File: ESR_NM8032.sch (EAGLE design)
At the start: 68 parts

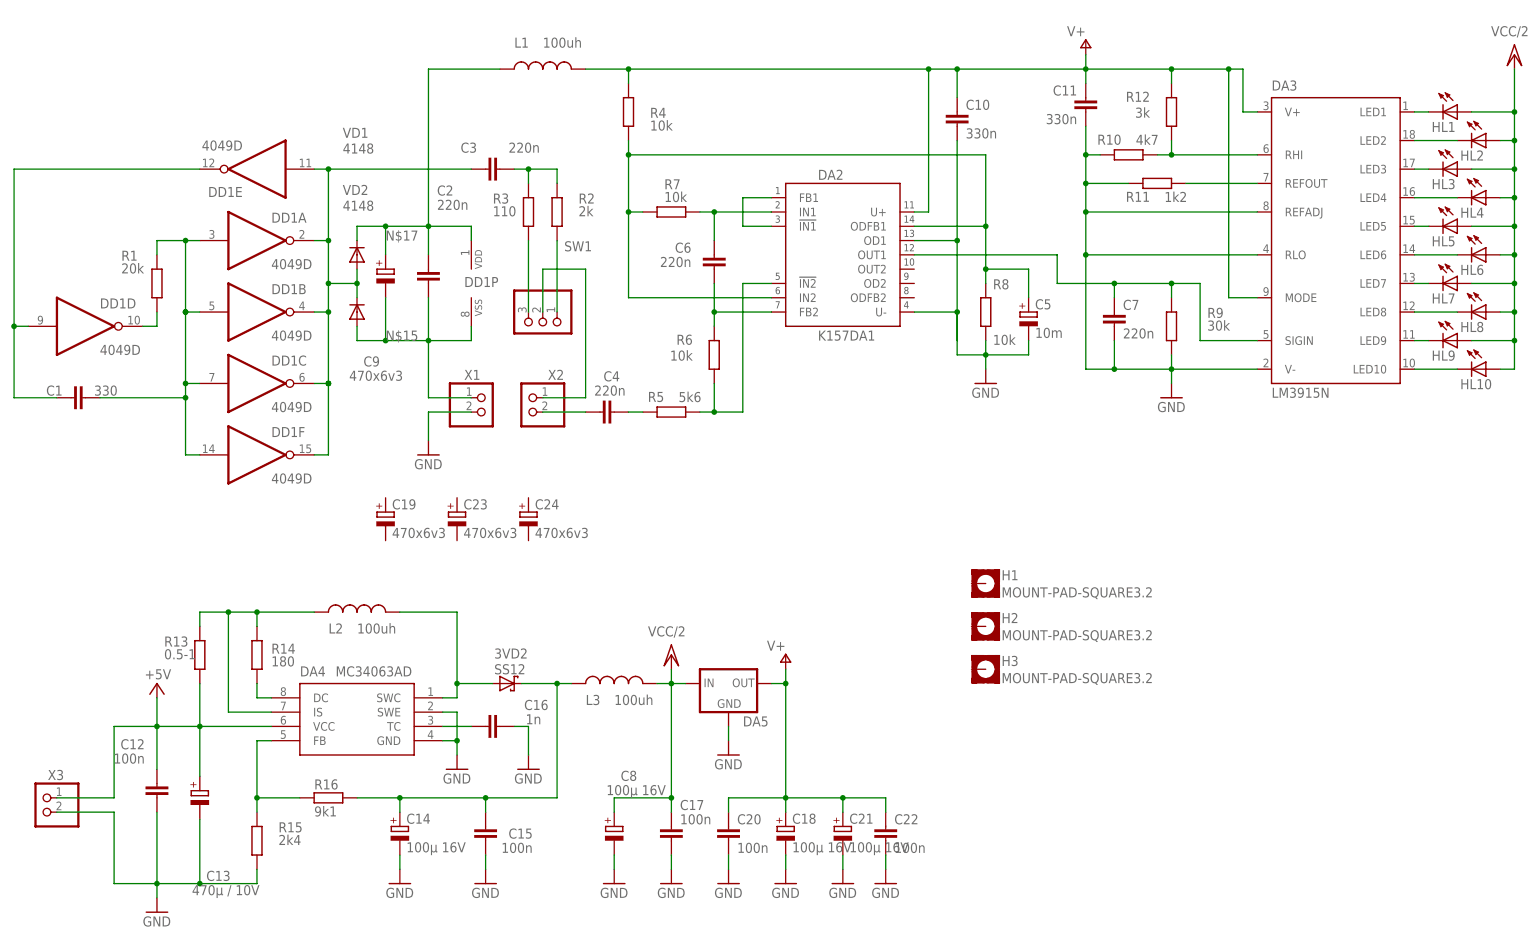
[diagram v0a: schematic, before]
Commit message: ..
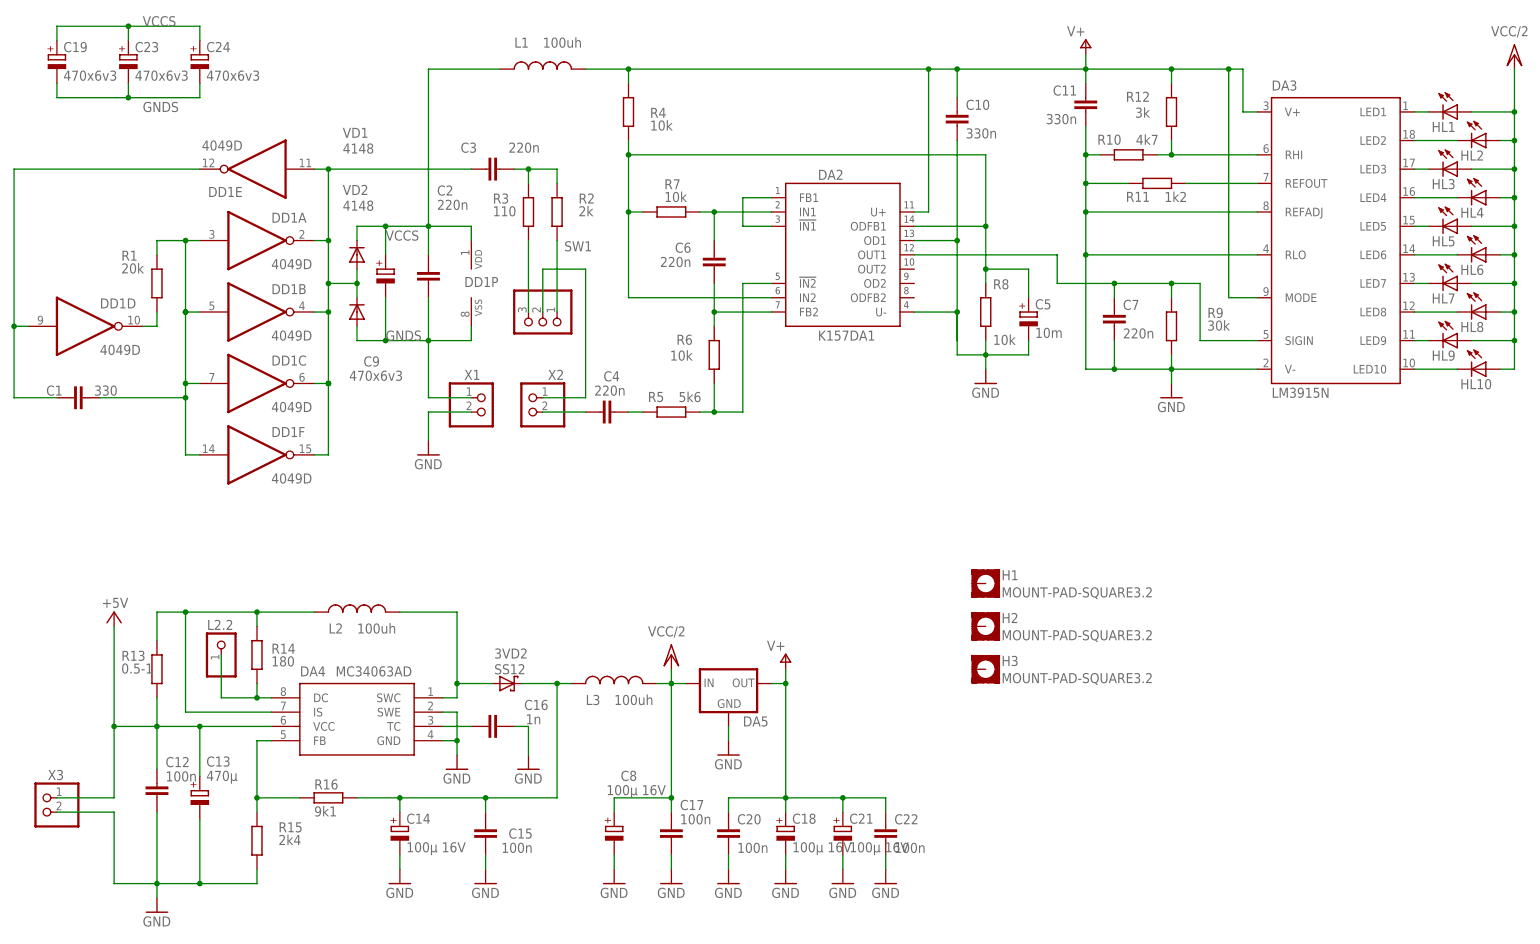
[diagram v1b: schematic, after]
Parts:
- added L2.2: (no value), pinhead:PINHD-1X1
- C13: value 470µ / 10V -> 470µ
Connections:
- removed net N$15: C2.2, C9.-, DD1P.VSS, VD2.A, X1.1
- removed net N$17: C2.1, C9.+, DD1P.VDD, L1.1, VD1.C
- new net GNDS: C19.-, C2.2, C23.-, C24.-, C9.-, DD1P.VSS, VD2.A, X1.1
- new net VCCS: C19.+, C2.1, C23.+, C24.+, C9.+, DD1P.VDD, L1.1, VD1.C
- net N$30: now also L2.2.1
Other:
- moved on the sheet: C19, C23, C24, R13
